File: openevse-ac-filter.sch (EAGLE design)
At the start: 7 parts

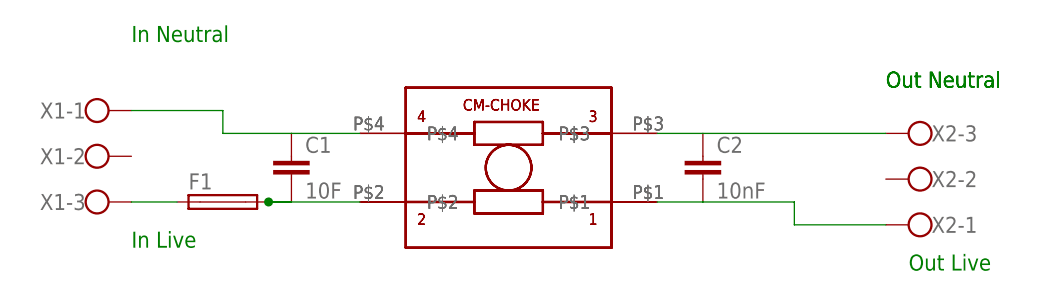
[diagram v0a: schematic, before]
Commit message: bump v2.1
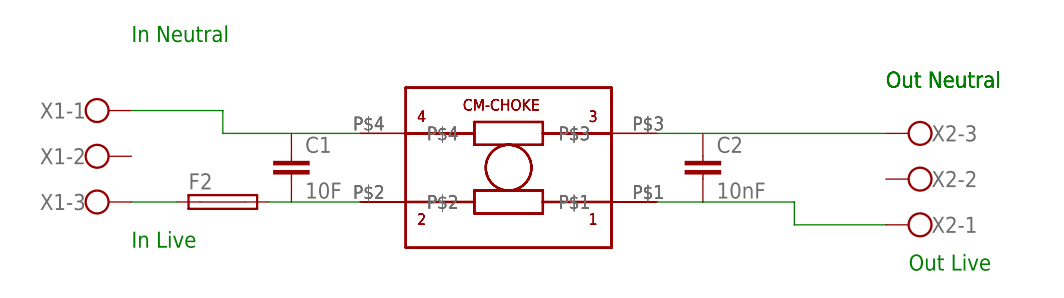
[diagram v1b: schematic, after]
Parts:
- removed F1: (no value), fuse:GSH15
- added F2: (no value), fuse-20mm:GSH15
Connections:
- net N$2: now also F2.2; no longer F1.2
- net N$5: now also F2.1; no longer F1.1
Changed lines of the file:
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@@
 <part name="X1" library="con-wago-500" library_urn="urn:adsk.eagle:library:195" deviceset="W237-103" device="" package3d_urn="urn:adsk.eagle:package:10691/1"/>
 <part name="X2" library="con-wago-500" library_urn="urn:adsk.eagle:library:195" deviceset="W237-103" device="" package3d_urn="urn:adsk.eagle:package:10691/1"/>
-<part name="F1" library="fuse" library_urn="urn:adsk.eagle:library:233" deviceset="GSH15" device="" package3d_urn="urn:adsk.eagle:package:14065/1"/>
+<part name="F2" library="fuse-20mm" deviceset="GSH15" device="" package3d_urn="urn:adsk.eagle:package:14065/1"/>
 </parts>
 <sheets>
@@
 <attribute name="NAME" x="81.28" y="75.311" size="1.778" layer="95"/>
 </instance>
-<instance part="F1" gate="1" x="2.54" y="68.58" smashed="yes">
+<instance part="F2" gate="1" x="2.54" y="68.58" smashed="yes">
 <attribute name="NAME" x="-1.27" y="69.977" size="1.778" layer="95"/>
 <attribute name="VALUE" x="-1.27" y="65.659" size="1.778" layer="96"/>
@@
 <pinref part="U$2" gate="G$1" pin="P$2"/>
 <pinref part="C1" gate="G$1" pin="2"/>
-<wire x1="7.62" y1="68.58" x2="17.78" y2="68.58" width="0.1524" layer="91"/>
-<pinref part="F1" gate="1" pin="2"/>
-<junction x="7.62" y="68.58"/>
+<wire x1="10.16" y1="68.58" x2="17.78" y2="68.58" width="0.1524" layer="91"/>
 <wire x1="7.62" y1="68.58" x2="10.16" y2="68.58" width="0.1524" layer="91"/>
+<pinref part="F2" gate="1" pin="2"/>
 </segment>
 </net>
@@
 <segment>
 <pinref part="X1" gate="-3" pin="KL"/>
-<pinref part="F1" gate="1" pin="1"/>
 <wire x1="-2.54" y1="68.58" x2="-7.62" y2="68.58" width="0.1524" layer="91"/>
+<pinref part="F2" gate="1" pin="1"/>
 </segment>
 </net>
